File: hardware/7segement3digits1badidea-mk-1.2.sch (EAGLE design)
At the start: 12 parts, among them IC1 MAX7219

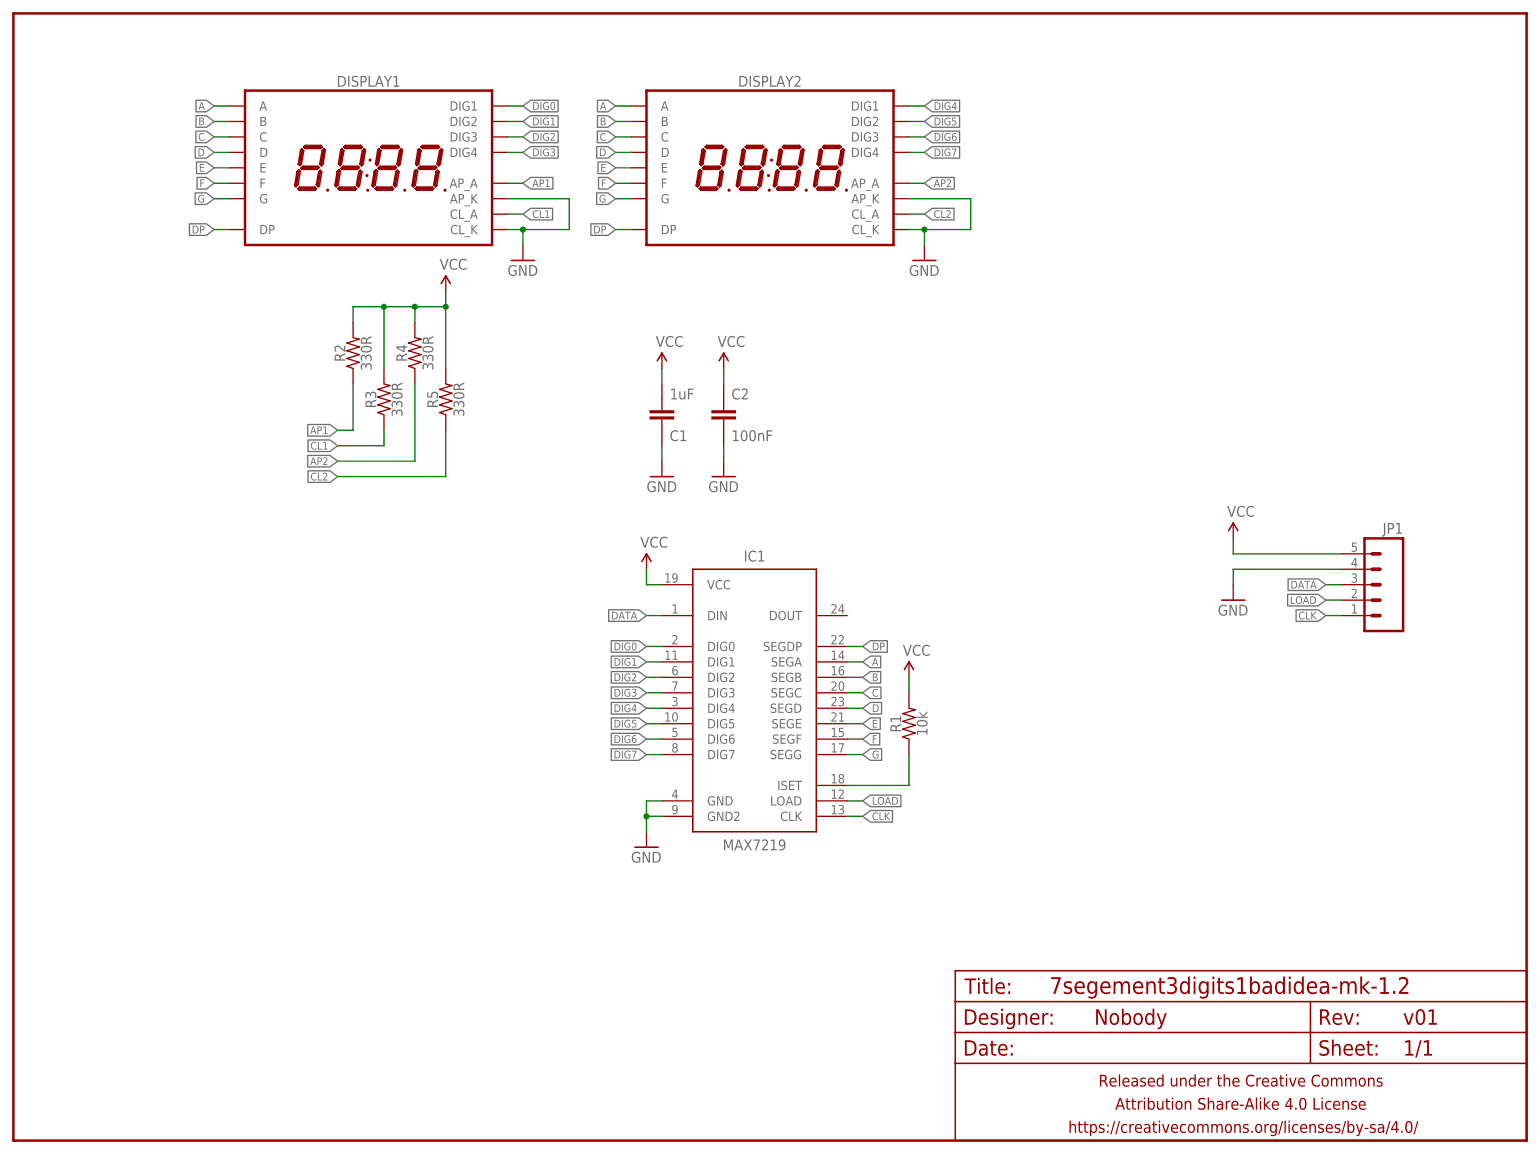
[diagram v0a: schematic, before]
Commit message: whooooole bunch of designs i apparently never committed
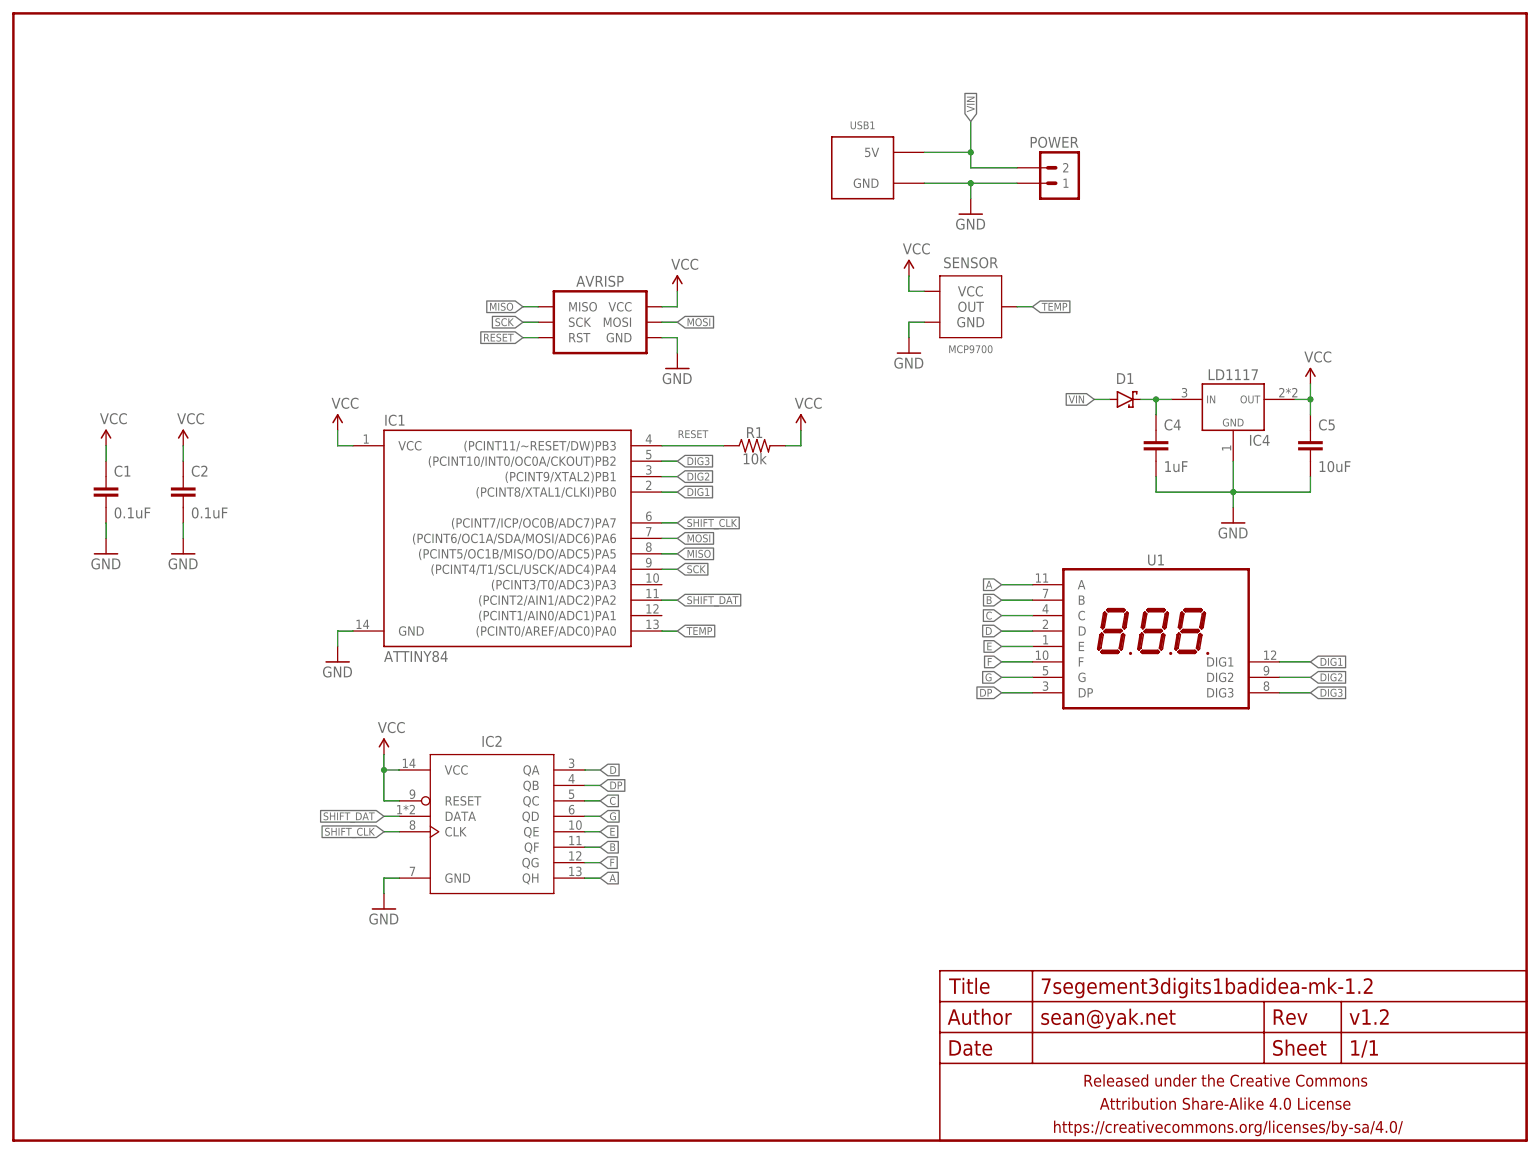
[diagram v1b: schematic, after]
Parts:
- removed DISPLAY1, DISPLAY2: 7SEG_4DIGIT_COLON_APOS, A_butts:7SEG_4DIGIT_COLON_APOS
- removed JP1: M05PTH, A_butts:M05PTH
- removed R2, R3, R4, R5: 330R, A_butts:RESISTORR0805
- added AVRISP: AVR_SPI_PRG_6TESTPOINTS, A_butts:AVR_SPI_PRG_6TESTPOINTS
- added C4: 1uF, A_butts:CAPACITOR-CERAMICC0805
- added C5: 10uF, A_butts:CAPACITOR-CERAMICC0805
- added D1: (no value), a_parts:DIODE-SCHOTTKYSOD123
- added IC2: 74HC164, a_parts:74164SOIC
- added IC4: LD1117, a_parts:VREG_1117SOT223
- added POWER: M02PTH-CENTERED-R+, A_butts:M02PTH-CENTERED-R+
- added SENSOR: MCP9700, a_parts:MCP9700TO-92-AMMO
- added U1: 7SEG_3DIGIT, a_parts:7SEG_3DIGIT
- added USB1: USB_AB_PWRONLY, A_butts:USB_AB_PWRONLY
- C1: value 1uF -> 0.1uF; device A_butts:CAPACITOR-CERAMICC0805 -> A_butts:CAPACITOR-CERAMICC0603
- C2: value 100nF -> 0.1uF; device A_butts:CAPACITOR-CERAMICC0805 -> A_butts:CAPACITOR-CERAMICC0603
- FRAME1: DESIGNER (none) -> sean@yak.net; VERSION (none) -> v1.2
- IC1: value MAX7219 -> ATTINY84; device A_butts:MAX7219SOIC-W -> A_butts:ATTINY84
- R1: device A_butts:RESISTORR0805 -> A_butts:RESISTORR0603
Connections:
- removed net AP1: DISPLAY1.AP_A, R2.1
- removed net AP2: DISPLAY2.AP_A, R4.1
- removed net CL1: DISPLAY1.CL_A, R3.1
- removed net CL2: DISPLAY2.CL_A, R5.1
- removed net CLK: IC1.CLK, JP1.1
- removed net DATA: IC1.DIN, JP1.3
- removed net DIG0: DISPLAY1.DIG1, IC1.DIG0
- removed net DIG4: DISPLAY2.DIG1, IC1.DIG4
- removed net DIG5: DISPLAY2.DIG2, IC1.DIG5
- removed net DIG6: DISPLAY2.DIG3, IC1.DIG6
- removed net DIG7: DISPLAY2.DIG4, IC1.DIG7
- removed net LOAD: IC1.LOAD, JP1.2
- removed net N$1: IC1.ISET, R1.1
- new net MISO: AVRISP.MISO, IC1.(PCINT5/OC1B/MISO/DO/ADC5)PA5
- new net MOSI: AVRISP.MOSI, IC1.(PCINT6/OC1A/SDA/MOSI/ADC6)PA6
- new net N$4: C4.1, D1.C, IC4.VIN
- new net RESET: AVRISP.RST, IC1.(PCINT11/~RESET/DW)PB3, R1.1
- new net SCK: AVRISP.SCK, IC1.(PCINT4/T1/SCL/USCK/ADC4)PA4
- new net SHIFT_CLK: IC1.(PCINT7/ICP/OC0B/ADC7)PA7, IC2.CLK
- new net SHIFT_DAT: IC1.(PCINT2/AIN1/ADC2)PA2, IC2.DATA
- new net TEMP: IC1.(PCINT0/AREF/ADC0)PA0, SENSOR.OUT
- new net VIN: D1.A, POWER.2, USB1.5V
- net A: now also IC2.QH, U1.A; no longer DISPLAY1.A, DISPLAY2.A, IC1.SEGA
- net B: now also IC2.QF, U1.B; no longer DISPLAY1.B, DISPLAY2.B, IC1.SEGB
- net C: now also IC2.QC, U1.C; no longer DISPLAY1.C, DISPLAY2.C, IC1.SEGC
- net D: now also IC2.QA, U1.D; no longer DISPLAY1.D, DISPLAY2.D, IC1.SEGD
- net DIG1: now also IC1.(PCINT8/XTAL1/CLKI)PB0, U1.DIG1; no longer DISPLAY1.DIG2, IC1.DIG1
- net DIG2: now also IC1.(PCINT9/XTAL2)PB1, U1.DIG2; no longer DISPLAY1.DIG3, IC1.DIG2
- net DIG3: now also IC1.(PCINT10/INT0/OC0A/CKOUT)PB2, U1.DIG3; no longer DISPLAY1.DIG4, IC1.DIG3
- net DP: now also IC2.QB, U1.DP; no longer DISPLAY1.DP, DISPLAY2.DP, IC1.SEGDP
- net E: now also IC2.QE, U1.E; no longer DISPLAY1.E, DISPLAY2.E, IC1.SEGE
- net F: now also IC2.QG, U1.F; no longer DISPLAY1.F, DISPLAY2.F, IC1.SEGF
- net G: now also IC2.QD, U1.G; no longer DISPLAY1.G, DISPLAY2.G, IC1.SEGG
- net GND: now also AVRISP.GND, C1.2, C4.2, C5.2, IC2.GND, IC4.GND, POWER.1, SENSOR.GND, USB1.GND; no longer C1.1, DISPLAY1.AP_K, DISPLAY1.CL_K, DISPLAY2.AP_K, DISPLAY2.CL_K, IC1.GND2, JP1.4
- net VCC: now also AVRISP.VCC, C1.1, C5.1, IC2.RESET, IC2.VCC, IC4.VOUT, SENSOR.VCC; no longer C1.2, JP1.5, R2.2, R3.2, R4.2, R5.2
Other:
- moved on the sheet: C1, C2, R1
